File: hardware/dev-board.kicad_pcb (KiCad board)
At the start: 2 copper layers, 6 parts, among them J1 Debug, J2 USB_C_Receptacle_USB2.0, U1 E73-2G4M08S1C

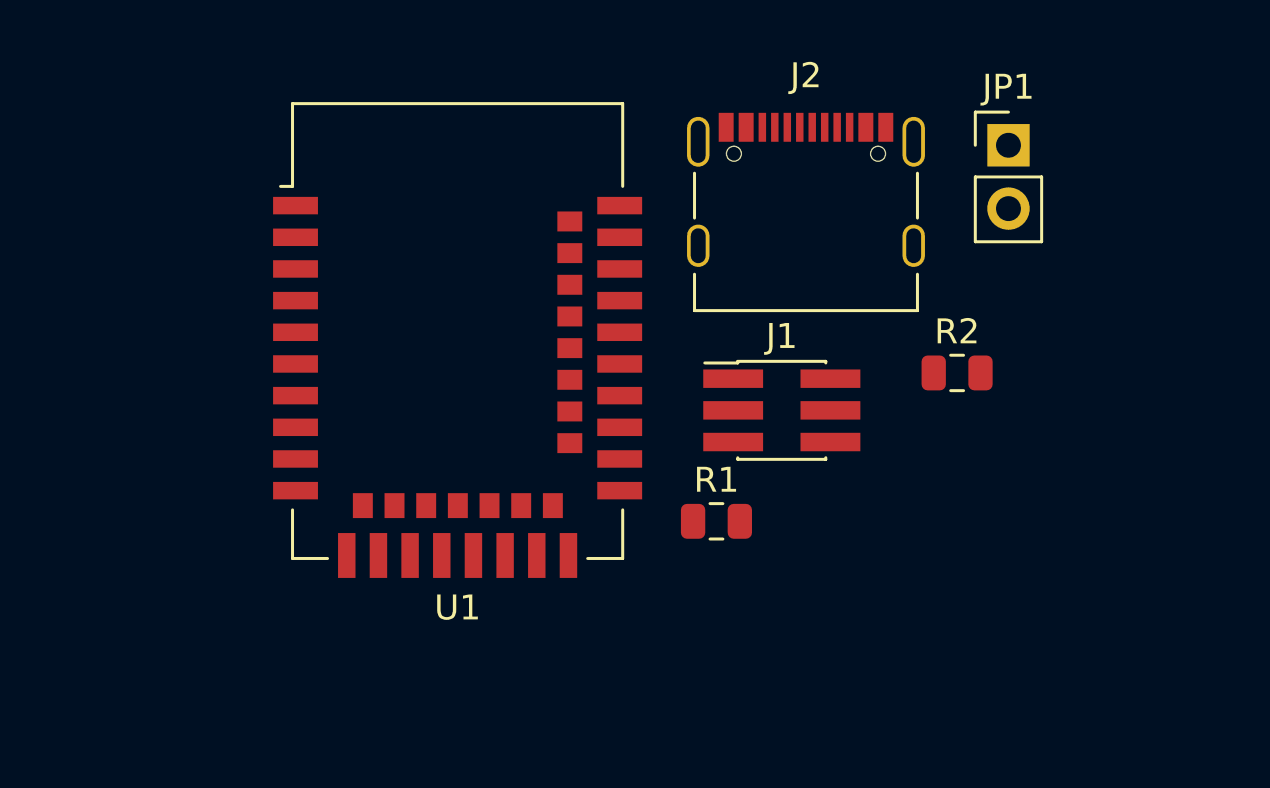
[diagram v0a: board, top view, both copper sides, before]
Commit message: Dev Board v1.0.0.0
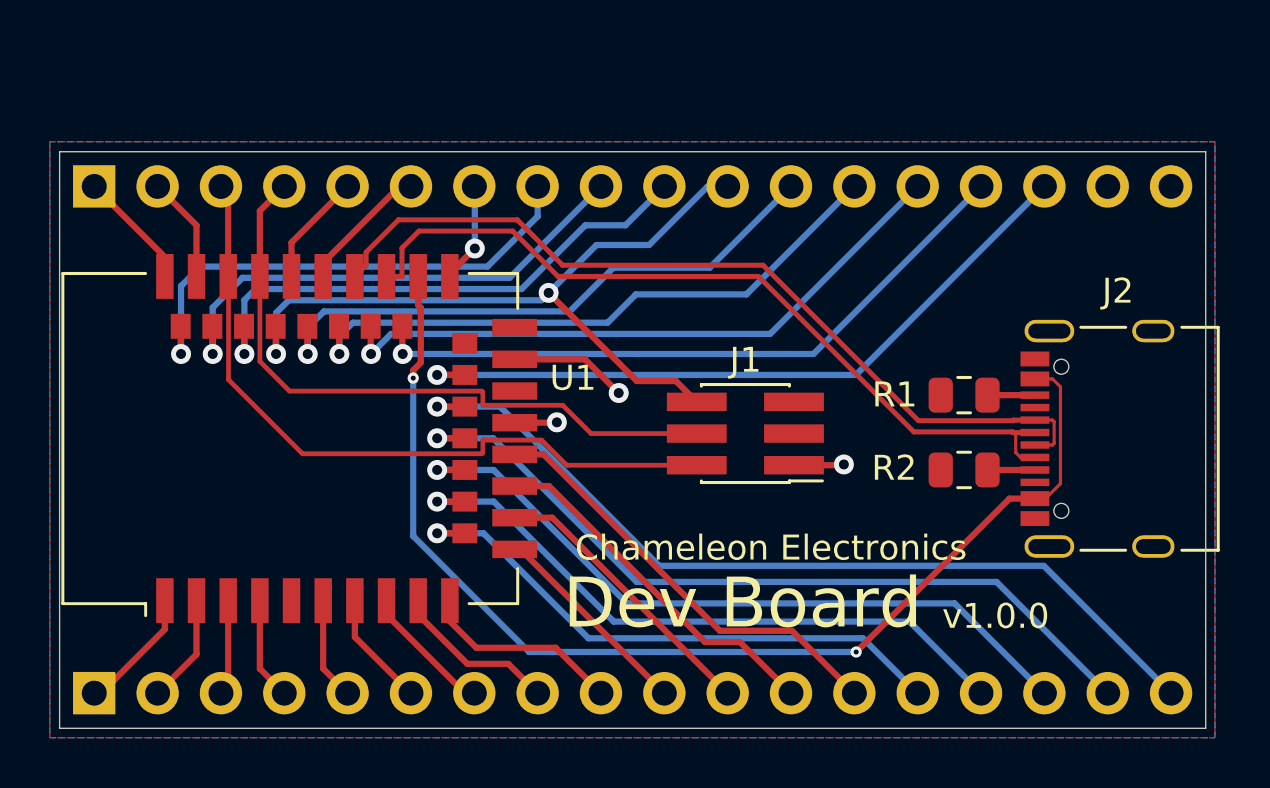
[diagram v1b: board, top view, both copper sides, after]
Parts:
- removed JP1: Jumper, Connector_PinHeader_2.54mm:PinHeader_1x02_P2.54mm_Vertical
- added J3: Conn_01x18_Male, Connector_PinHeader_2.54mm:PinHeader_1x18_P2.54mm_Vertical, B.Cu at (123.9, 88.5)
- added J4: Conn_01x18_Male, Connector_PinHeader_2.54mm:PinHeader_1x18_P2.54mm_Vertical, B.Cu at (123.9, 108.8)
- moved J2 15.4 mm to (164.1, 98.6), turned to 90 degrees
- moved R1 11.1 mm to (158.8, 96.8), turned to 180 degrees
- moved U1 7.91 mm to (131.8, 98.6), turned to 90 degrees
- moved R2 3.90 mm to (158.8, 99.8), turned to 180 degrees
- moved J1 1.73 mm to (150.0, 98.4), turned to 180 degrees
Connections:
- net Net-(J2-PadA6) renamed /D+
- net Net-(J2-PadA7) renamed /D-
- J2 pad A4: Net-(J2-PadA4) -> /VBUS
- J2 pad A9: Net-(J2-PadA4) -> /VBUS
- J2 pad B4: Net-(J2-PadA4) -> /VBUS
- J2 pad B9: Net-(J2-PadA4) -> /VBUS
- U1 pad 1: Net-(U1-Pad1) -> /P1.11
- U1 pad 10: Net-(U1-Pad10) -> /P0.30
- U1 pad 11: Net-(U1-Pad11) -> /P0.00
- U1 pad 12: Net-(U1-Pad12) -> /P0.26
- U1 pad 13: Net-(U1-Pad13) -> /P0.11
- U1 pad 14: Net-(U1-Pad14) -> /P0.06
- U1 pad 15: Net-(U1-Pad15) -> /P0.05
- U1 pad 16: Net-(U1-Pad16) -> /P0.08
- U1 pad 17: Net-(U1-Pad17) -> /P1.09
- U1 pad 18: Net-(U1-Pad18) -> /P0.04
- U1 pad 19: /VDD -> +3V3
- U1 pad 2: Net-(U1-Pad2) -> /P1.10
- U1 pad 20: Net-(U1-Pad20) -> /P0.12
- U1 pad 22: Net-(U1-Pad22) -> /P0.07
- U1 pad 23: /VDDH -> +3V3
- U1 pad 26: Net-(U1-Pad26) -> /P0.18
- U1 pad 28: Net-(U1-Pad28) -> /P0.15
- U1 pad 3: Net-(U1-Pad3) -> /P0.03
- U1 pad 30: Net-(U1-Pad30) -> /P0.17
- U1 pad 32: Net-(U1-Pad32) -> /P0.20
- U1 pad 33: Net-(U1-Pad33) -> /P0.13
- U1 pad 34: Net-(U1-Pad34) -> /P0.22
- U1 pad 35: Net-(U1-Pad35) -> /P0.24
- U1 pad 38: Net-(U1-Pad38) -> /P1.02
- U1 pad 4: Net-(U1-Pad4) -> /P0.28
- U1 pad 40: Net-(U1-Pad40) -> /P1.04
- U1 pad 41: Net-(U1-Pad41) -> /P0.09
- U1 pad 42: Net-(U1-Pad42) -> /P1.06
- U1 pad 43: Net-(U1-Pad43) -> /P0.10
- U1 pad 6: Net-(U1-Pad6) -> /P1.13
- U1 pad 7: Net-(U1-Pad7) -> /P0.02
- U1 pad 8: Net-(U1-Pad8) -> /P0.29
- U1 pad 9: Net-(U1-Pad9) -> /P0.31
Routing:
- net /VBUS: track 0.00 -> 46.3 mm, vias 0 -> 2
- net /P0.12: track 0.00 -> 35.3 mm, vias 0 -> 1
- net /D+: track 0.00 -> 34.3 mm
- net /D-: track 0.00 -> 33.2 mm
- net /P0.04: track 0.00 -> 32.2 mm, vias 0 -> 1
- net /SWO: track 0.00 -> 30.7 mm, vias 0 -> 2
- net /P0.08: track 0.00 -> 29.2 mm, vias 0 -> 1
- net /SWDCLK: track 0.00 -> 28.8 mm
- net /P0.07: track 0.00 -> 28.6 mm, vias 0 -> 1
- net /P0.15: track 0.00 -> 27.1 mm, vias 0 -> 1
- net /SWDIO: track 0.00 -> 26.4 mm
- net /P0.06: track 0.00 -> 26.1 mm, vias 0 -> 1
- net /P0.17: track 0.00 -> 25.8 mm, vias 0 -> 1
- net /P0.20: track 0.00 -> 25.0 mm, vias 0 -> 1
- net /P0.22: track 0.00 -> 23.9 mm, vias 0 -> 1
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- added copper zone on B.Cu, net +3V3
- added copper zone on F.Cu, net GND
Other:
- board outline added: 46 x 23.1 mm
- net class Default: clearance 0.2 -> 0.127; trace_width 0.25 -> 0.127; via_dia 0.8 -> 0.45; via_drill 0.4 -> 0.2
- rule trace_clearance: 0.2 -> 0.127
- rule trace_min: 0.2 -> 0.127
- rule via_min_drill: 0.3 -> 0.2
- rule via_min_size: 0.4 -> 0.45
- board text added: "Chameleon Electronics"
- board text added: "Dev Board"
- board text added: "v1.0.0"
